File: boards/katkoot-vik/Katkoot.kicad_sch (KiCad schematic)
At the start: 24 parts, among them J11 Conn_01x18, SW16 SW_Push, SW17 SW_Push, SW34 Rotary_Encoder_Switch, SW6 SW_Push, SW7 SW_Push, SW8 SW_Push, U1 TCR2EF19,LM(CT, U2 PMW3360DM-T2QU, U2 xiao-ble

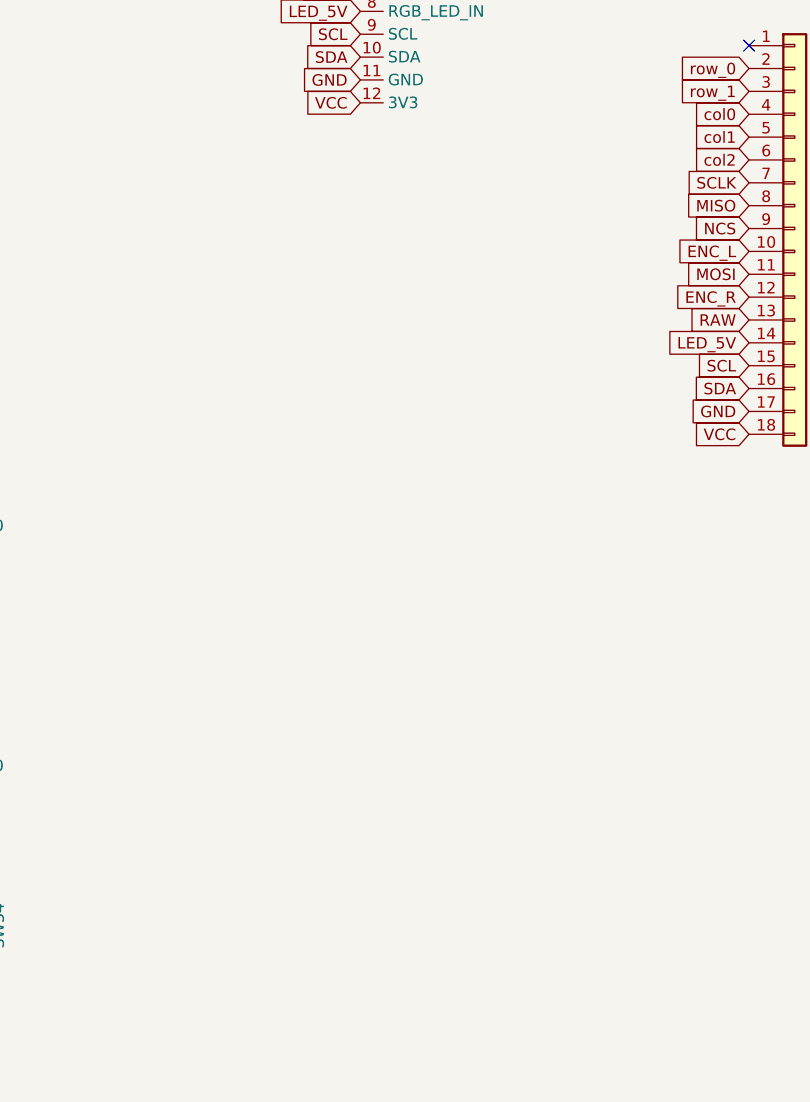
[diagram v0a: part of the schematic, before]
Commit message: VIK Katkoot
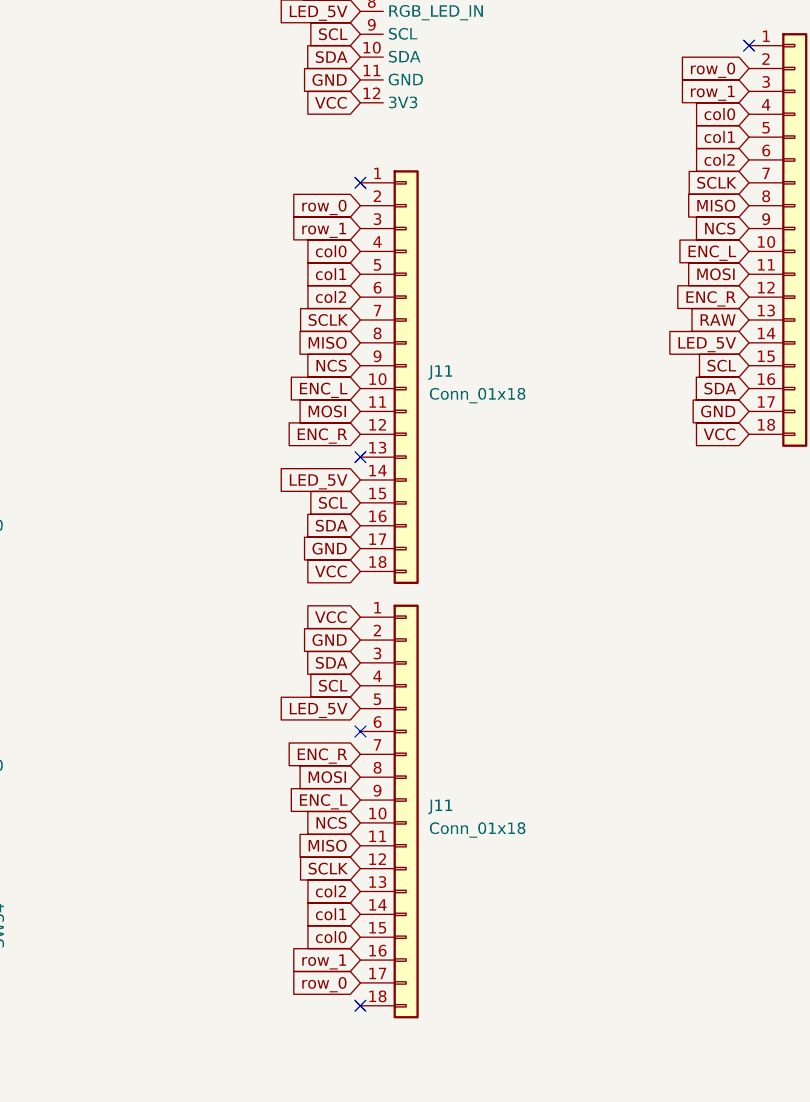
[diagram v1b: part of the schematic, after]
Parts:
- added J11 (x2): Conn_01x18, Alaa:FPC-SMD_FPC05018-09200-.5mm-rev, symbol Connector_Generic:Conn_01x18
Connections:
- net ENC_L: now also J11.10 (Pin_10), J11.9 (Pin_9)
- net ENC_R: now also J11.12 (Pin_12), J11.7 (Pin_7)
- net GND: now also J11.17 (Pin_17), J11.2 (Pin_2)
- net LED_5V: now also J11.14 (Pin_14), J11.5 (Pin_5)
- net MISO: now also J11.11 (Pin_11), J11.8 (Pin_8)
- net MOSI: now also J11.11 (Pin_11), J11.8 (Pin_8)
- net NCS: now also J11.10 (Pin_10), J11.9 (Pin_9)
- net SCL: now also J11.15 (Pin_15), J11.4 (Pin_4)
- net SCLK: now also J11.12 (Pin_12), J11.7 (Pin_7)
- net SDA: now also J11.16 (Pin_16), J11.3 (Pin_3)
- net VCC: now also J11.1 (Pin_1), J11.18 (Pin_18)
- net col0: now also J11.15 (Pin_15), J11.4 (Pin_4)
- net col1: now also J11.14 (Pin_14), J11.5 (Pin_5)
- net col2: now also J11.13 (Pin_13), J11.6 (Pin_6)
- net row_0: now also J11.17 (Pin_17), J11.2 (Pin_2)
- net row_1: now also J11.16 (Pin_16), J11.3 (Pin_3)
- no-connect marks 11 -> 15
